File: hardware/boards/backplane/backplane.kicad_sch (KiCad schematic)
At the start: 7 parts, among them J1 DC_IN_SCREW_TERMINAL, J2 XT30U(2+2)-F.G.B_SLOT1, J3 XT30U(2+2)-F.G.B_SLOT2, J4 XT30U(2+2)-F.G.B_SLOT3, J5 XT30U(2+2)-F.G.B_SLOT4, J6 XT30U(2+2)-F.G.B_SLOT5, J7 XT30U(2+2)-F.G.B_SLOT6

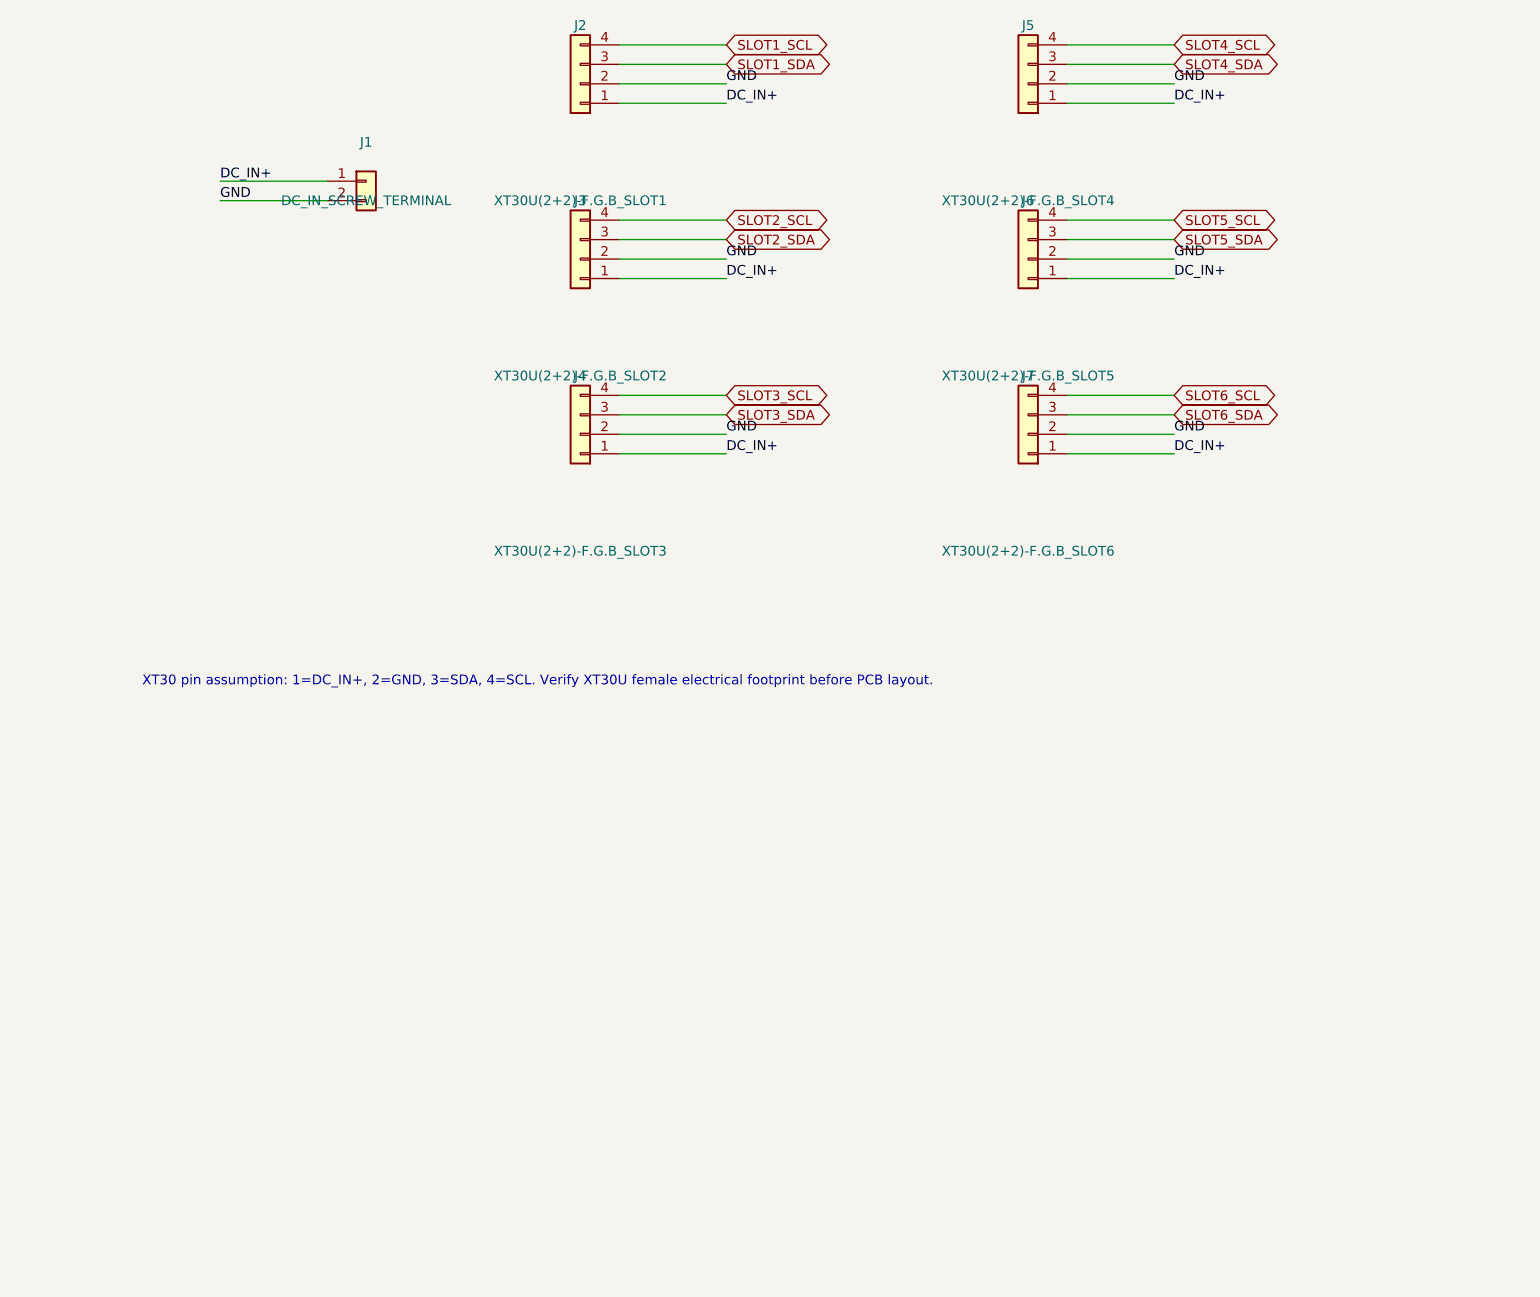
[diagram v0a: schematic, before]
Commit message: Checkpoint
_sigh_
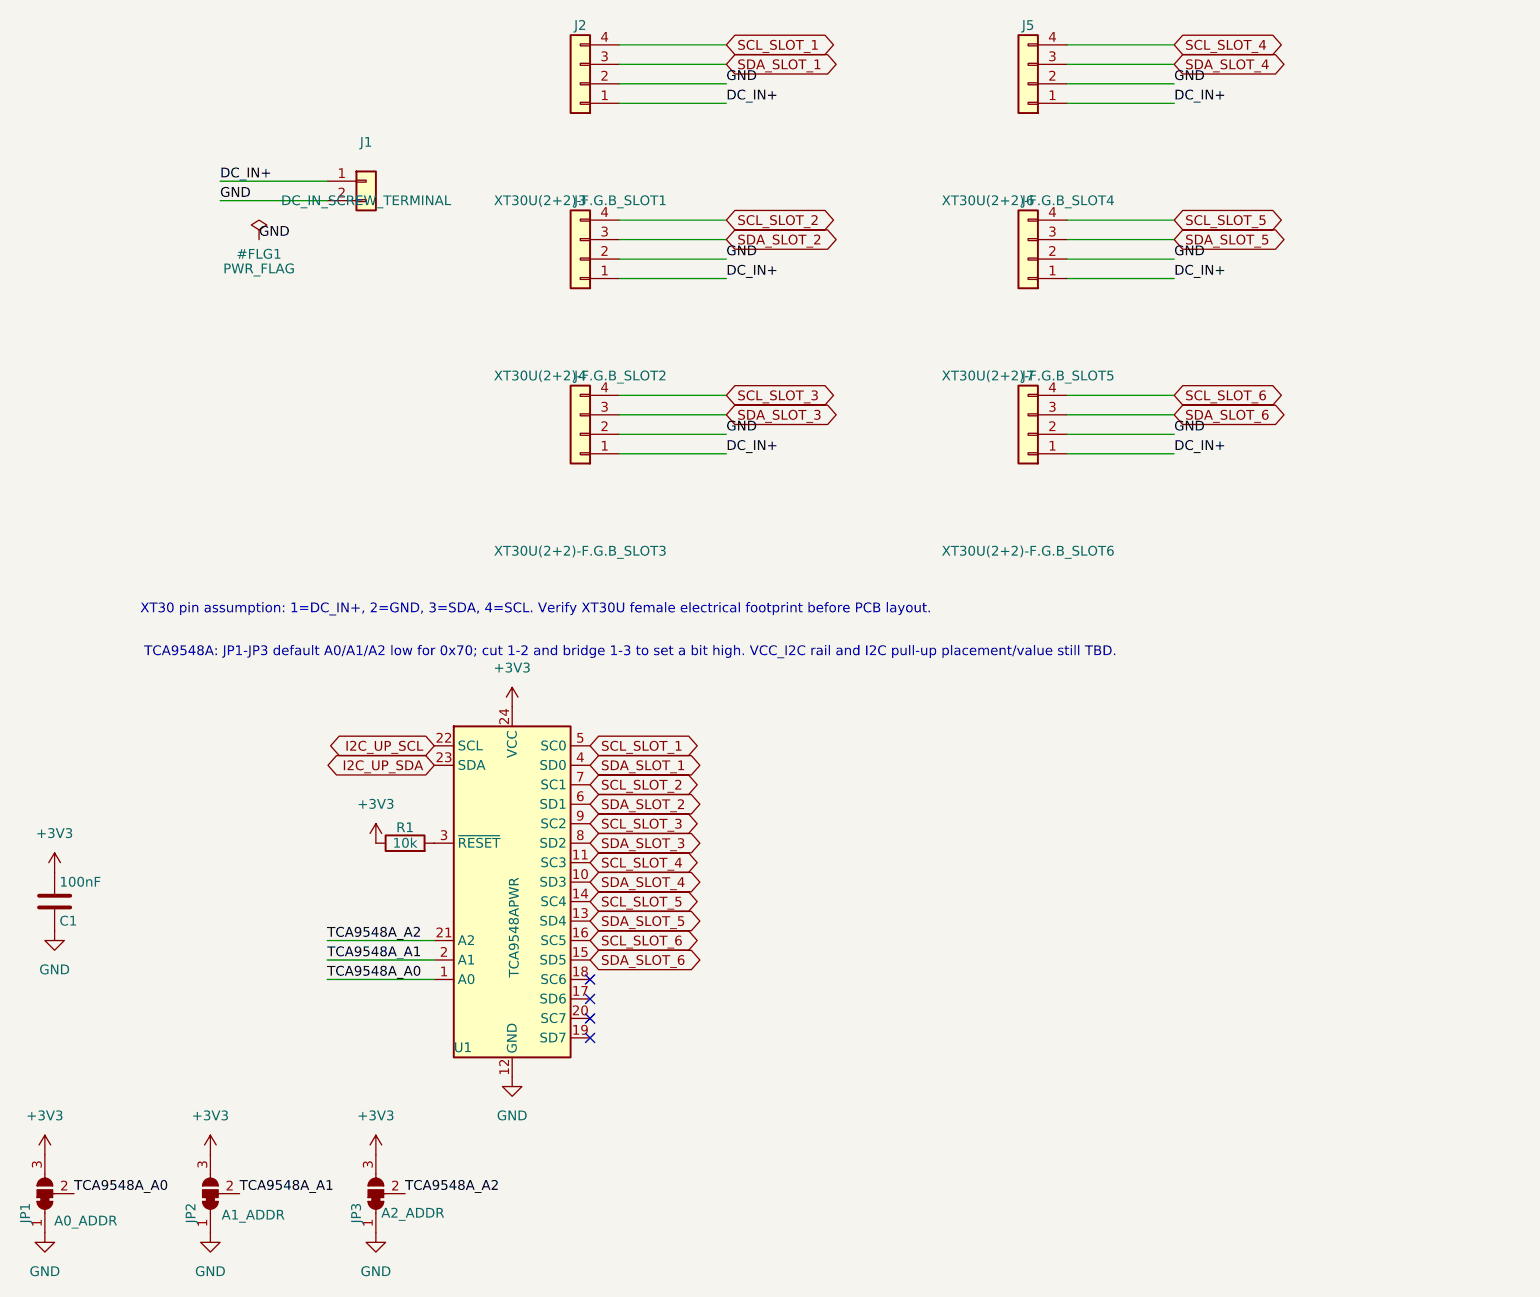
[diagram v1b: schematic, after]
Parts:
- added C1: 100nF, Capacitor_SMD:C_0603_1608Metric, symbol Device:C
- added JP1: A0_ADDR, Jumper:SolderJumper-3_P1.3mm_Bridged12_Pad1.0x1.5mm, symbol Jumper:SolderJumper_3_Bridged12
- added JP2: A1_ADDR, Jumper:SolderJumper-3_P1.3mm_Bridged12_Pad1.0x1.5mm, symbol Jumper:SolderJumper_3_Bridged12
- added JP3: A2_ADDR, Jumper:SolderJumper-3_P1.3mm_Bridged12_Pad1.0x1.5mm, symbol Jumper:SolderJumper_3_Bridged12
- added R1: 10k, Resistor_SMD:R_0603_1608Metric, symbol Device:R
- added U1: TCA9548APWR, Package_SO:TSSOP-24_4.4x7.8mm_P0.65mm, symbol Interface_Expansion:TCA9548APWR
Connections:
- net GND: now also C1.2, JP1.1 (A), JP2.1 (A), JP3.1 (A), U1.12 (GND)
- net SLOT1_SCL renamed SCL_SLOT_1
- net SCL_SLOT_1: now also U1.5 (SC0)
- net SLOT1_SDA renamed SDA_SLOT_1
- net SDA_SLOT_1: now also U1.4 (SD0)
- net SLOT2_SCL renamed SCL_SLOT_2
- net SCL_SLOT_2: now also U1.7 (SC1)
- net SLOT2_SDA renamed SDA_SLOT_2
- net SDA_SLOT_2: now also U1.6 (SD1)
- net SLOT3_SCL renamed SCL_SLOT_3
- net SCL_SLOT_3: now also U1.9 (SC2)
- net SLOT3_SDA renamed SDA_SLOT_3
- net SDA_SLOT_3: now also U1.8 (SD2)
- net SLOT4_SCL renamed SCL_SLOT_4
- net SCL_SLOT_4: now also U1.11 (SC3)
- net SLOT4_SDA renamed SDA_SLOT_4
- net SDA_SLOT_4: now also U1.10 (SD3)
- net SLOT5_SCL renamed SCL_SLOT_5
- net SCL_SLOT_5: now also U1.14 (SC4)
- net SLOT5_SDA renamed SDA_SLOT_5
- net SDA_SLOT_5: now also U1.13 (SD4)
- net SLOT6_SCL renamed SCL_SLOT_6
- net SCL_SLOT_6: now also U1.16 (SC5)
- net SLOT6_SDA renamed SDA_SLOT_6
- net SDA_SLOT_6: now also U1.15 (SD5)
- new net: R1.2, U1.3 (~{RESET})
- new net +3V3: C1.1, JP1.3 (B), JP2.3 (B), JP3.3 (B), R1.1, U1.24 (VCC)
- new net I2C_UP_SCL: U1.22 (SCL)
- new net I2C_UP_SDA: U1.23 (SDA)
- new net TCA9548A_A0: JP1.2 (C), U1.1 (A0)
- new net TCA9548A_A1: JP2.2 (C), U1.2 (A1)
- new net TCA9548A_A2: JP3.2 (C), U1.21 (A2)
- no-connect marks 0 -> 4
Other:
- note added: "TCA9548A: JP1-JP3 default A0/A1/A2 low for 0x70; cut 1-2 and bridge 1-3 to set a bit high. VCC_I2C rail and I2C pull-up placement/value still TBD."
